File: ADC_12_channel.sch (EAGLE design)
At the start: 163 parts, among them IC1 LM317BD2T, IC2 LM317BD2T, K1 691131710003, K2 691101710002, K3 691101710002, K4 691101710002, K5 691101710002, K6 691101710002, K7 691101710002, K8 691101710002, K9 691101710002, U1 AD7864ASZ-1, U10 TL082D, U12 V_REG_317SMD, U2 AD7864ASZ-1, U3 TL082D, U4 TL082D, U5 TL082D, U6 TL082D, U7 TL082D, U8 TL082D, U9 TL082D, X1 QTE-040

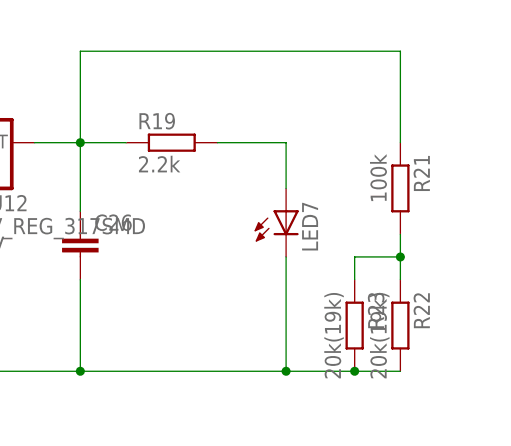
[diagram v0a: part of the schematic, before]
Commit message: Supply Finally sorted out!
arranging supply components
Working on realigning resistors of input stage
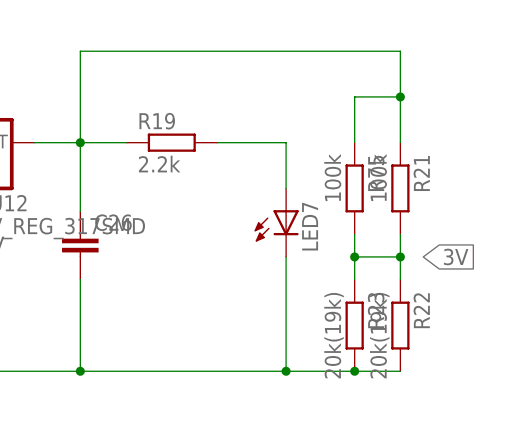
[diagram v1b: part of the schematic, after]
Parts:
- added R75: 100k, rcl:R-EU_R1206
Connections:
- removed net 0.8V: R21.2, R22.1, R23.1
- new net 3V: R21.2, R22.1, R23.1, R75.2
- net VCC_5+: now also R75.1
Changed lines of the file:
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@@
 <grid distance="0.1" unitdist="inch" unit="inch" style="lines" multiple="1" display="no" altdistance="0.01" altunitdist="inch" altunit="inch"/>
 <layers>
-<layer number="1" name="Top" color="4" fill="1" visible="yes" active="no"/>
-<layer number="2" name="Route2" color="1" fill="3" visible="yes" active="no"/>
-<layer number="3" name="Route3" color="4" fill="3" visible="yes" active="no"/>
-<layer number="4" name="Route4" color="1" fill="4" visible="yes" active="no"/>
-<layer number="5" name="Route5" color="4" fill="4" visible="yes" active="no"/>
-<layer number="6" name="Route6" color="1" fill="8" visible="yes" active="no"/>
-<layer number="7" name="Route7" color="4" fill="8" visible="yes" active="no"/>
-<layer number="8" name="Route8" color="1" fill="2" visible="yes" active="no"/>
-<layer number="9" name="Route9" color="4" fill="2" visible="yes" active="no"/>
-<layer number="10" name="Route10" color="1" fill="7" visible="yes" active="no"/>
-<layer number="11" name="Route11" color="4" fill="7" visible="yes" active="no"/>
-<layer number="12" name="Route12" color="1" fill="5" visible="yes" active="no"/>
-<layer number="13" name="Route13" color="4" fill="5" visible="yes" active="no"/>
-<layer number="14" name="Route14" color="1" fill="6" visible="yes" active="no"/>
-<layer number="15" name="Route15" color="4" fill="6" visible="yes" active="no"/>
-<layer number="16" name="Bottom" color="1" fill="1" visible="yes" active="no"/>
-<layer number="17" name="Pads" color="2" fill="1" visible="yes" active="no"/>
-<layer number="18" name="Vias" color="2" fill="1" visible="yes" active="no"/>
-<layer number="19" name="Unrouted" color="6" fill="1" visible="yes" active="no"/>
-<layer number="20" name="Dimension" color="15" fill="1" visible="yes" active="no"/>
-<layer number="21" name="tPlace" color="7" fill="1" visible="yes" active="no"/>
-<layer number="22" name="bPlace" color="7" fill="1" visible="yes" active="no"/>
-<layer number="23" name="tOrigins" color="15" fill="1" visible="yes" active="no"/>
-<layer number="24" name="bOrigins" color="15" fill="1" visible="yes" active="no"/>
-<layer number="25" name="tNames" color="7" fill="1" visible="yes" active="no"/>
-<layer number="26" name="bNames" color="7" fill="1" visible="yes" active="no"/>
-<layer number="27" name="tValues" color="7" fill="1" visible="yes" active="no"/>
-<layer number="28" name="bValues" color="7" fill="1" visible="yes" active="no"/>
+<layer number="1" name="Top" color="4" fill="1" visible="no" active="no"/>
+<layer number="2" name="Route2" color="1" fill="3" visible="no" active="no"/>
+<layer number="3" name="Route3" color="4" fill="3" visible="no" active="no"/>
+<layer number="4" name="Route4" color="1" fill="4" visible="no" active="no"/>
+<layer number="5" name="Route5" color="4" fill="4" visible="no" active="no"/>
+<layer number="6" name="Route6" color="1" fill="8" visible="no" active="no"/>
+<layer number="7" name="Route7" color="4" fill="8" visible="no" active="no"/>
+<layer number="8" name="Route8" color="1" fill="2" visible="no" active="no"/>
+<layer number="9" name="Route9" color="4" fill="2" visible="no" active="no"/>
+<layer number="10" name="Route10" color="1" fill="7" visible="no" active="no"/>
+<layer number="11" name="Route11" color="4" fill="7" visible="no" active="no"/>
+<layer number="12" name="Route12" color="1" fill="5" visible="no" active="no"/>
+<layer number="13" name="Route13" color="4" fill="5" visible="no" active="no"/>
+<layer number="14" name="Route14" color="1" fill="6" visible="no" active="no"/>
+<layer number="15" name="Route15" color="4" fill="6" visible="no" active="no"/>
+<layer number="16" name="Bottom" color="1" fill="1" visible="no" active="no"/>
+<layer number="17" name="Pads" color="2" fill="1" visible="no" active="no"/>
+<layer number="18" name="Vias" color="2" fill="1" visible="no" active="no"/>
+<layer number="19" name="Unrouted" color="6" fill="1" visible="no" active="no"/>
+<layer number="20" name="Dimension" color="15" fill="1" visible="no" active="no"/>
+<layer number="21" name="tPlace" color="7" fill="1" visible="no" active="no"/>
+<layer number="22" name="bPlace" color="7" fill="1" visible="no" active="no"/>
+<layer number="23" name="tOrigins" color="15" fill="1" visible="no" active="no"/>
+<layer number="24" name="bOrigins" color="15" fill="1" visible="no" active="no"/>
+<layer number="25" name="tNames" color="7" fill="1" visible="no" active="no"/>
+<layer number="26" name="bNames" color="7" fill="1" visible="no" active="no"/>
+<layer number="27" name="tValues" color="7" fill="1" visible="no" active="no"/>
+<layer number="28" name="bValues" color="7" fill="1" visible="no" active="no"/>
 <layer number="29" name="tStop" color="7" fill="3" visible="no" active="no"/>
 <layer number="30" name="bStop" color="7" fill="6" visible="no" active="no"/>
@@
 <layer number="35" name="tGlue" color="7" fill="4" visible="no" active="no"/>
 <layer number="36" name="bGlue" color="7" fill="5" visible="no" active="no"/>
-<layer number="37" name="tTest" color="7" fill="1" visible="yes" active="no"/>
-<layer number="38" name="bTest" color="7" fill="1" visible="yes" active="no"/>
+<layer number="37" name="tTest" color="7" fill="1" visible="no" active="no"/>
+<layer number="38" name="bTest" color="7" fill="1" visible="no" active="no"/>
 <layer number="39" name="tKeepout" color="4" fill="11" visible="no" active="no"/>
 <layer number="40" name="bKeepout" color="1" fill="11" visible="no" active="no"/>
@@
 <layer number="44" name="Drills" color="7" fill="1" visible="no" active="no"/>
 <layer number="45" name="Holes" color="7" fill="1" visible="no" active="no"/>
-<layer number="46" name="Milling" color="3" fill="1" visible="yes" active="no"/>
-<layer number="47" name="Measures" color="7" fill="1" visible="yes" active="no"/>
-<layer number="48" name="Document" color="7" fill="1" visible="yes" active="no"/>
-<layer number="49" name="Reference" color="7" fill="1" visible="yes" active="no"/>
-<layer number="50" name="dxf" color="7" fill="1" visible="yes" active="no"/>
-<layer number="51" name="tDocu" color="7" fill="1" visible="yes" active="no"/>
-<layer number="52" name="bDocu" color="7" fill="1" visible="yes" active="no"/>
-<layer number="53" name="tGND_GNDA" color="7" fill="9" visible="yes" active="no"/>
-<layer number="54" name="bGND_GNDA" color="1" fill="9" visible="yes" active="no"/>
-<layer number="56" name="wert" color="7" fill="1" visible="yes" active="no"/>
-<layer number="57" name="tCAD" color="7" fill="1" visible="yes" active="no"/>
-<layer number="59" name="tCarbon" color="7" fill="1" visible="yes" active="no"/>
-<layer number="60" name="bCarbon" color="7" fill="1" visible="yes" active="no"/>
+<layer number="46" name="Milling" color="3" fill="1" visible="no" active="no"/>
+<layer number="47" name="Measures" color="7" fill="1" visible="no" active="no"/>
+<layer number="48" name="Document" color="7" fill="1" visible="no" active="no"/>
+<layer number="49" name="Reference" color="7" fill="1" visible="no" active="no"/>
+<layer number="50" name="dxf" color="7" fill="1" visible="no" active="no"/>
+<layer number="51" name="tDocu" color="7" fill="1" visible="no" active="no"/>
+<layer number="52" name="bDocu" color="7" fill="1" visible="no" active="no"/>
+<layer number="53" name="tGND_GNDA" color="7" fill="9" visible="no" active="no"/>
+<layer number="54" name="bGND_GNDA" color="1" fill="9" visible="no" active="no"/>
+<layer number="56" name="wert" color="7" fill="1" visible="no" active="no"/>
+<layer number="57" name="tCAD" color="7" fill="1" visible="no" active="no"/>
+<layer number="59" name="tCarbon" color="7" fill="1" visible="no" active="no"/>
+<layer number="60" name="bCarbon" color="7" fill="1" visible="no" active="no"/>
 <layer number="90" name="Modules" color="5" fill="1" visible="yes" active="yes"/>
 <layer number="91" name="Nets" color="2" fill="1" visible="yes" active="yes"/>
@@
 <part name="IC2" library="v-reg" deviceset="LM317?*" device="BD2T"/>
 <part name="R74" library="resistor" deviceset="R-EU_" device="M1206" value="0"/>
+<part name="R75" library="rcl" deviceset="R-EU_" device="R1206" value="100k"/>
 </parts>
 <sheets>
@@
 <instance part="IC2" gate="G$1" x="617.22" y="274.32"/>
 <instance part="R74" gate="G$1" x="-33.02" y="63.5" rot="R180"/>
+<instance part="R75" gate="G$1" x="731.52" y="276.86" rot="R270"/>
 </instances>
 <busses>
@@
 <pinref part="R21" gate="G$1" pin="1"/>
 <wire x1="701.04" y1="292.1" x2="736.6" y2="292.1" width="0.1524" layer="91"/>
-<wire x1="736.6" y1="292.1" x2="736.6" y2="281.94" width="0.1524" layer="91"/>
+<wire x1="736.6" y1="292.1" x2="736.6" y2="287.02" width="0.1524" layer="91"/>
 <pinref part="U12" gate="G$1" pin="OUT"/>
-</segment>
-</net>
-<net name="0.8V" class="0">
+<pinref part="R75" gate="G$1" pin="1"/>
+<wire x1="736.6" y1="287.02" x2="736.6" y2="281.94" width="0.1524" layer="91"/>
+<wire x1="731.52" y1="281.94" x2="731.52" y2="287.02" width="0.1524" layer="91"/>
+<wire x1="731.52" y1="287.02" x2="736.6" y2="287.02" width="0.1524" layer="91"/>
+<junction x="736.6" y="287.02"/>
+</segment>
+</net>
+<net name="3V" class="0">
 <segment>
 <pinref part="R21" gate="G$1" pin="2"/>
@@
 <wire x1="731.52" y1="266.7" x2="731.52" y2="269.24" width="0.1524" layer="91"/>
 <wire x1="731.52" y1="269.24" x2="736.6" y2="269.24" width="0.1524" layer="91"/>
-</segment>
-</net>
+<pinref part="R75" gate="G$1" pin="2"/>
+<wire x1="731.52" y1="271.78" x2="731.52" y2="269.24" width="0.1524" layer="91"/>
+<junction x="731.52" y="269.24"/>
+<label x="739.14" y="269.24" size="1.778" layer="95" xref="yes"/>
+</segment>
+</net>
